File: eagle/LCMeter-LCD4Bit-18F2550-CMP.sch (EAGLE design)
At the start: 35 parts, among them IC1 PIC18F2550-I/SP-COMP-B-V, J1 HD44780-4BITLCD44780-8P, J2 PIC-UART, J3 PIC-ICSP, J4 J4, J5 CONN-2P2P/V, J7 CONN-2P2P/V, K2 DS2Y, Q1 20MHz, SW1 PB-1P-1T, T1 BC547

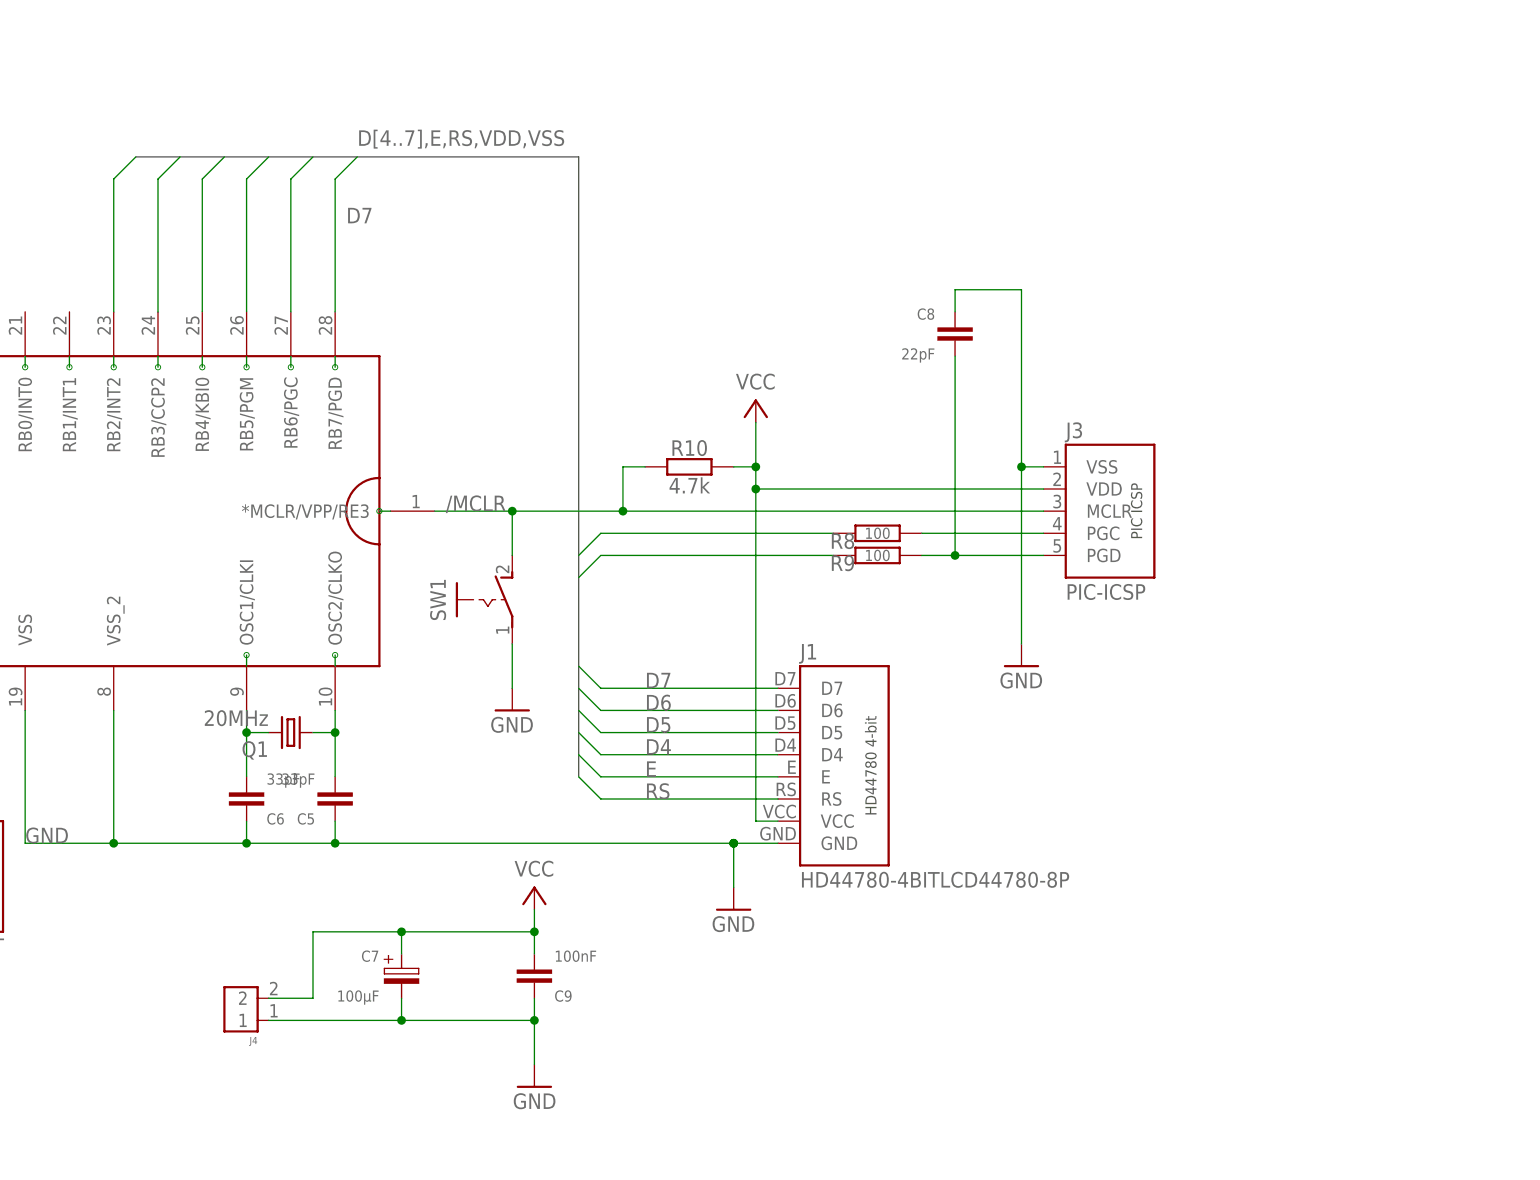
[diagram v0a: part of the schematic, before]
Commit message: ...
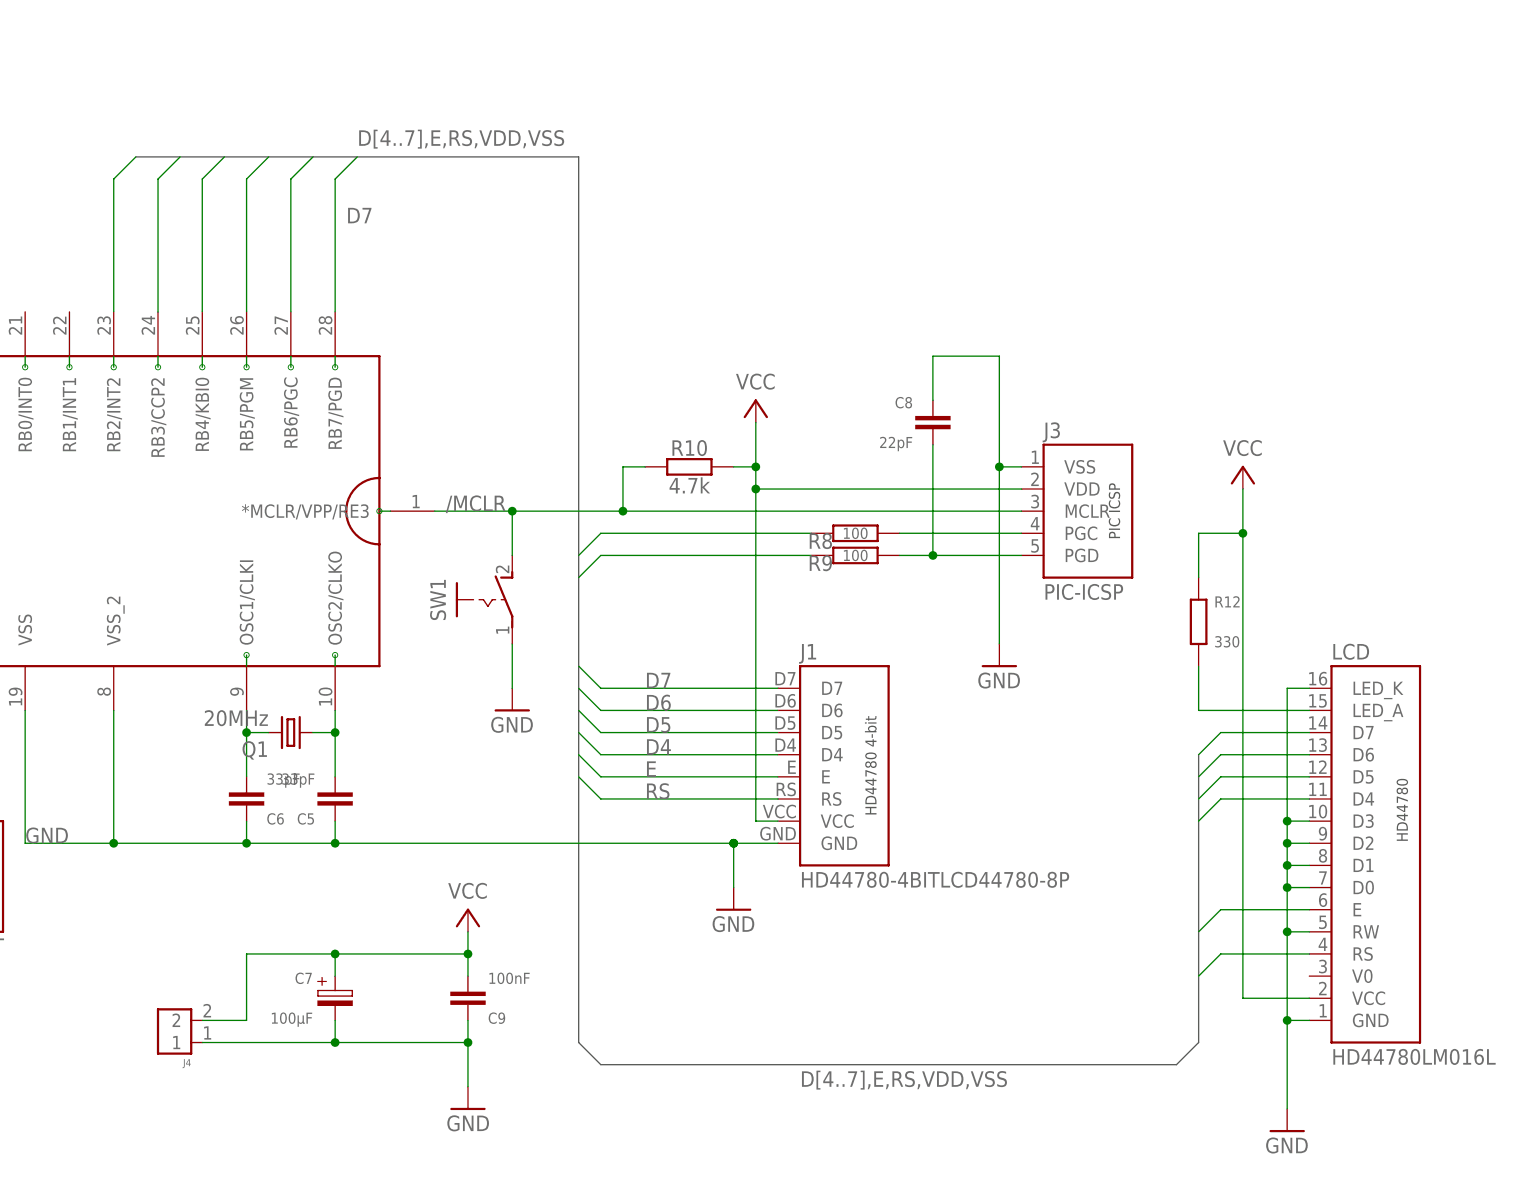
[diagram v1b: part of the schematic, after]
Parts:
- added LCD: HD44780LM016L, lcd:HD44780LM016L
- added R12: 330, r:R0202/7
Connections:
- new net N$5: LCD.LED_A, R12.1
- net D4: now also LCD.D4
- net D5: now also LCD.D5
- net D6: now also LCD.D6
- net D7: now also LCD.D7
- net E: now also LCD.E
- net GND: now also LCD.D0, LCD.D1, LCD.D2, LCD.D3, LCD.GND, LCD.LED_K, LCD.RW
- net RS: now also LCD.RS
- net VCC: now also LCD.VCC, R12.2
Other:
- moved on the sheet: C7, C8, C9, J3, J4, R8, R9
